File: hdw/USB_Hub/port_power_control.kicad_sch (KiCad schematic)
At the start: 12 parts

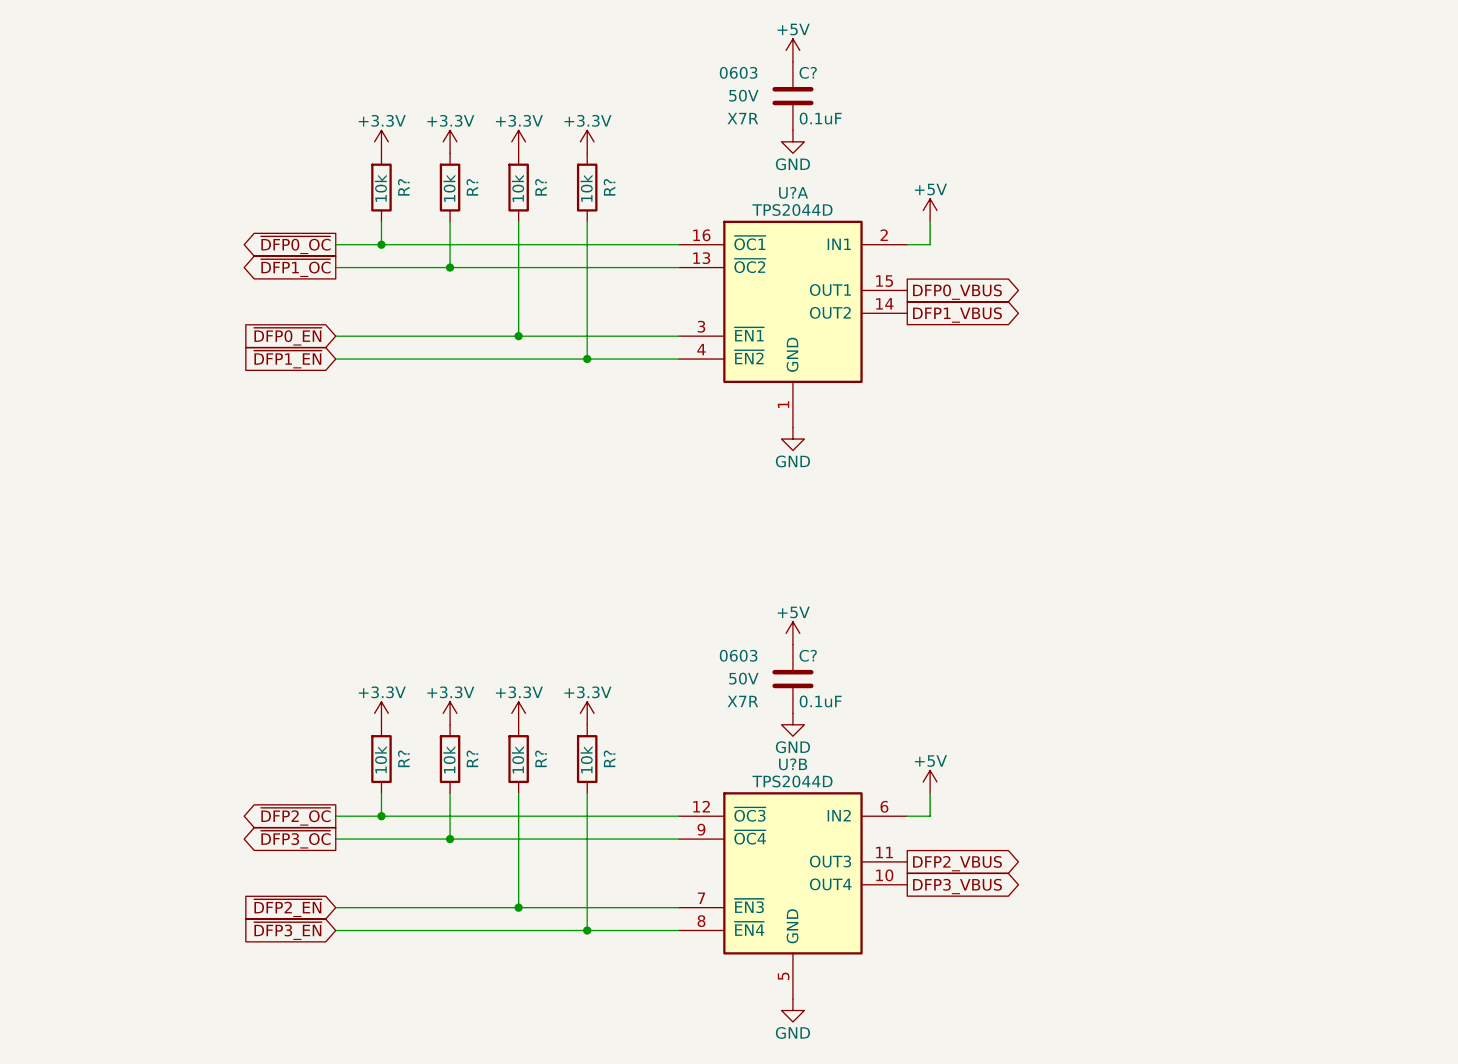
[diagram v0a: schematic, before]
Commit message: lots of schematic progress
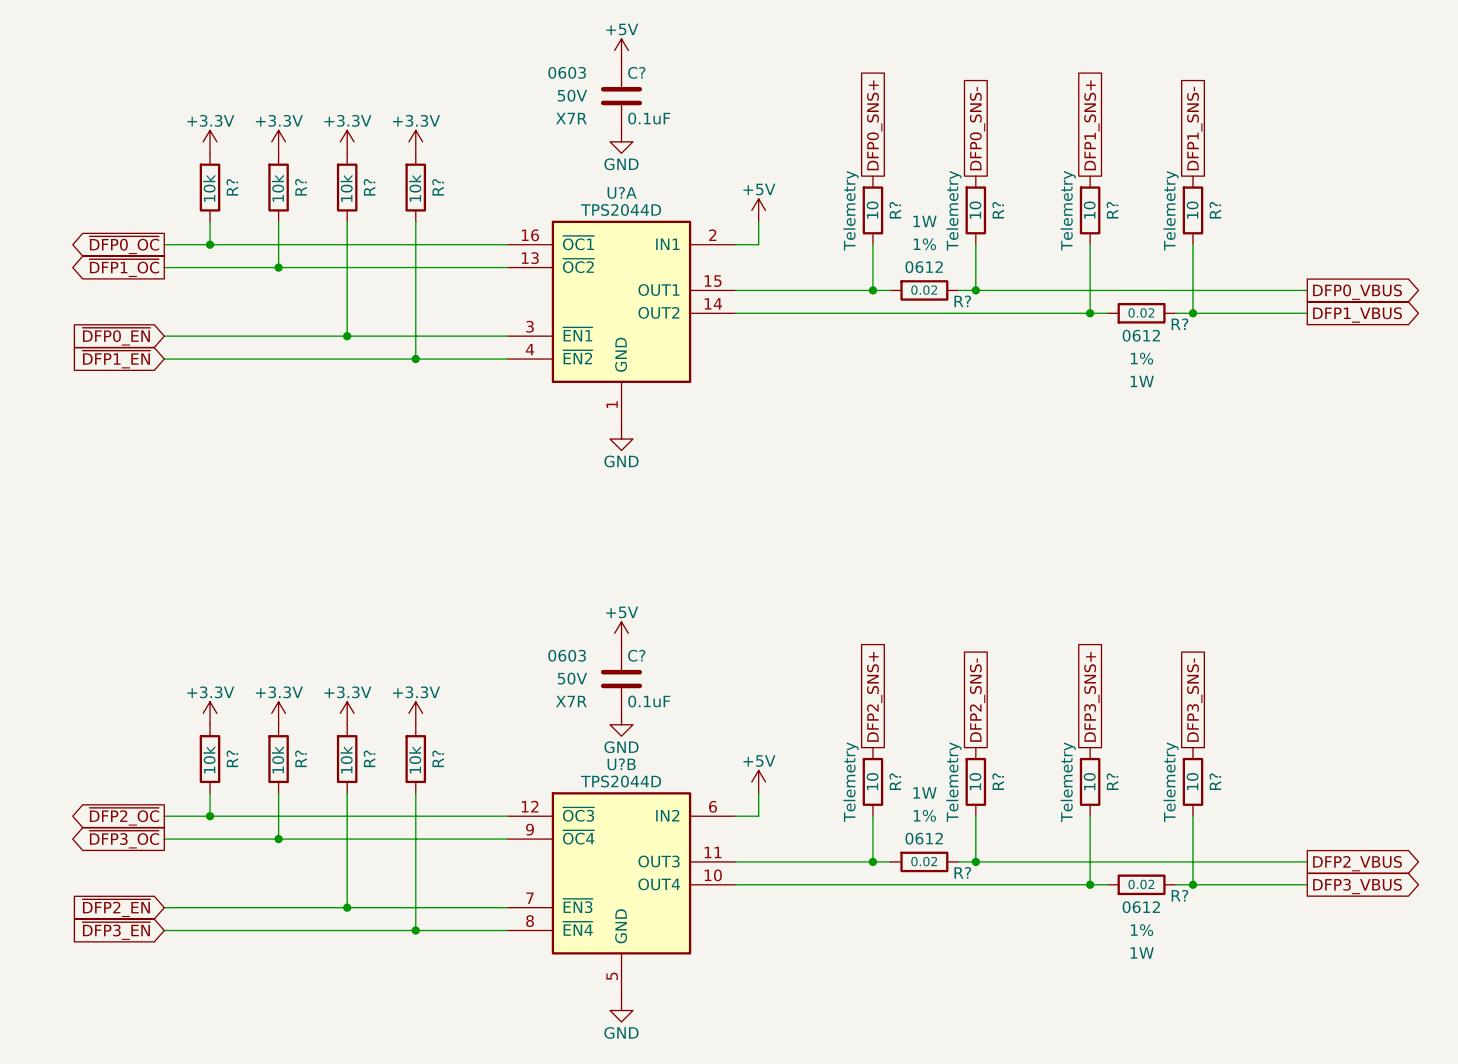
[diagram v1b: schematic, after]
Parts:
- added R? (x8): 10, Resistors_SMD:R_0402, symbol Custom_Library:R_Custom
- added R? (x4): 0.02, Resistors_SMD:R_0612, symbol Custom_Library:R_Custom
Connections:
- net DFP0_VBUS: now also R?.2, R?.2; no longer U?.15 (OUT1)
- net DFP1_VBUS: now also R?.2, R?.2; no longer U?.14 (OUT2)
- net DFP2_VBUS: now also R?.2, R?.2; no longer U?.11 (OUT3)
- net DFP3_VBUS: now also R?.2, R?.2; no longer U?.10 (OUT4)
- new net: R?.1, R?.2, U?.10 (OUT4)
- new net: R?.1, R?.2, U?.14 (OUT2)
- new net: R?.1, R?.2, U?.11 (OUT3)
- new net: R?.1, R?.2, U?.15 (OUT1)
- new net DFP0_SNS+: R?.1
- new net DFP0_SNS-: R?.1
- new net DFP1_SNS+: R?.1
- new net DFP1_SNS-: R?.1
- new net DFP2_SNS+: R?.1
- new net DFP2_SNS-: R?.1
- new net DFP3_SNS+: R?.1
- new net DFP3_SNS-: R?.1
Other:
- company: (none) -> Drew Maatman
- title: (none) -> USB Hub
- moved on the sheet: C?, R?, U?A, U?B
